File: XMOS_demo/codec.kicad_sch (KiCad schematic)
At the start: 1 part, among them U2 CS4271

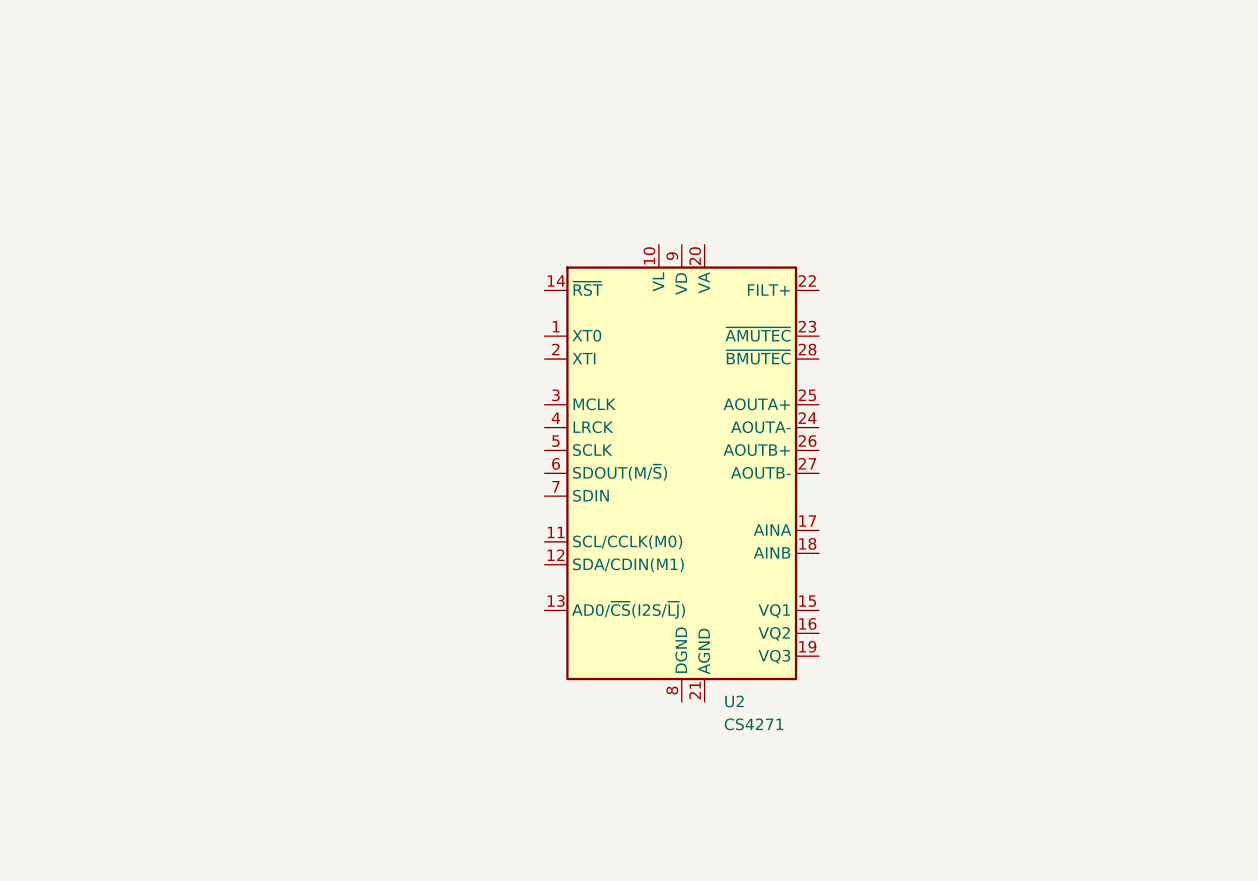
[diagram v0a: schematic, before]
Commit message: Lots of sch work
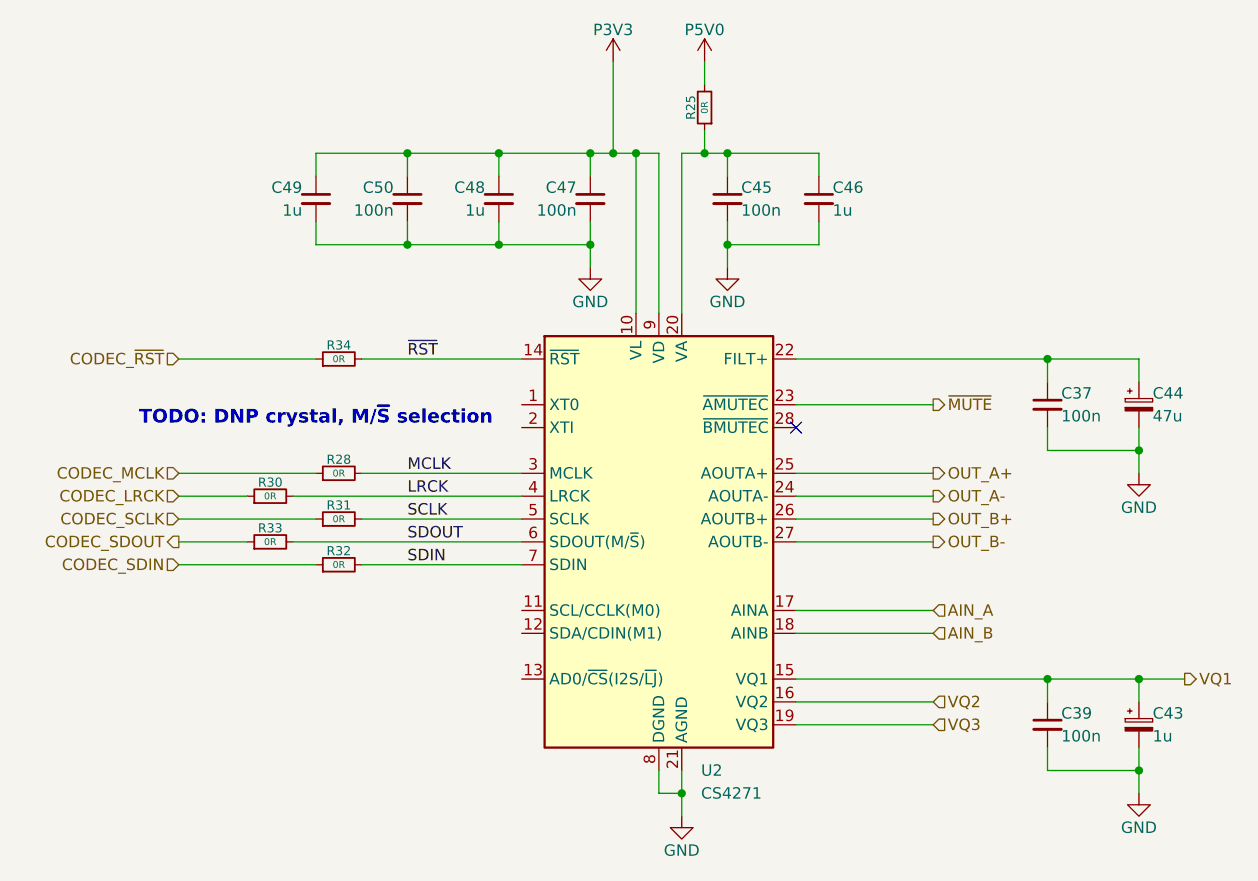
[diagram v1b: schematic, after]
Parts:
- added C37, C39, C45, C47, C50: 100n, Capacitor_SMD:C_0603_1608Metric, symbol Device:C_Small
- added C43: 1u, Capacitor_SMD:CP_Elec_4x5.4, symbol Device:C_Polarized_Small
- added C44: 47u, Capacitor_SMD:CP_Elec_6.3x5.7, symbol Device:C_Polarized_Small
- added C46, C48, C49: 1u, Capacitor_SMD:C_0603_1608Metric, symbol Device:C_Small
- added R25, R28, R30, R31, R32, R33, R34: 0R, Resistor_SMD:R_0603_1608Metric, symbol Device:R_Small
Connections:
- net P3V3: now reaches U2.10 (VL)
- net P3V3: now also U2.9 (VD), C47.1, C48.1, C49.1, C50.1
- net ~{RST}: now reaches U2.14 (~{RST})
- net ~{RST}: now also R34.2
- net VQ1: now reaches U2.15 (VQ1)
- net VQ1: now also C39.1, C43.1
- net VQ2: now reaches U2.16 (VQ2)
- net AIN_A: now reaches U2.17 (AINA)
- net AIN_B: now reaches U2.18 (AINB)
- net VQ3: now reaches U2.19 (VQ3)
- net at U2.20 (VA): now also C45.1, C46.1, R25.1
- net GND: now reaches U2.21 (AGND)
- net GND: now also U2.8 (DGND), C37.2, C39.2, C43.2, C44.2, C45.2, C46.2, C47.2, C48.2, C49.2, C50.2
- net at U2.22 (FILT+): now also C37.1, C44.1
- net ~{MUTE}: now reaches U2.23 (~{AMUTEC})
- net OUT_A-: now reaches U2.24 (AOUTA-)
- net OUT_A+: now reaches U2.25 (AOUTA+)
- net OUT_B+: now reaches U2.26 (AOUTB+)
- net OUT_B-: now reaches U2.27 (AOUTB-)
- net MCLK: now reaches U2.3 (MCLK)
- net MCLK: now also R28.2
- net LRCK: now reaches U2.4 (LRCK)
- net LRCK: now also R30.2
- net SCLK: now reaches U2.5 (SCLK)
- net SCLK: now also R31.2
- net SDOUT: now reaches U2.6 (SDOUT(M/~{S}))
- net SDOUT: now also R33.2
- net SDIN: now reaches U2.7 (SDIN)
- net SDIN: now also R32.2
- new net CODEC_LRCK: R30.1
- new net CODEC_MCLK: R28.1
- new net CODEC_SCLK: R31.1
- new net CODEC_SDIN: R32.1
- new net CODEC_SDOUT: R33.1
- new net CODEC_~{RST}: R34.1
- new net P5V0: R25.2
- no-connect marks 0 -> 1
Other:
- note added: "TODO: DNP crystal, M/~{S} selection"
- moved on the sheet: U2
